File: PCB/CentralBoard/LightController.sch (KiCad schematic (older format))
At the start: 29 parts, among them P1 CONN_01X03, P2 CONN_01X10, P3 CONN_01X03, P4 CONN_01X10, P5 CONN_01X03, SW1 SW_DIP_x06, U1 LM317_3PinPackage, U2 NCP551, U3 PCA9685

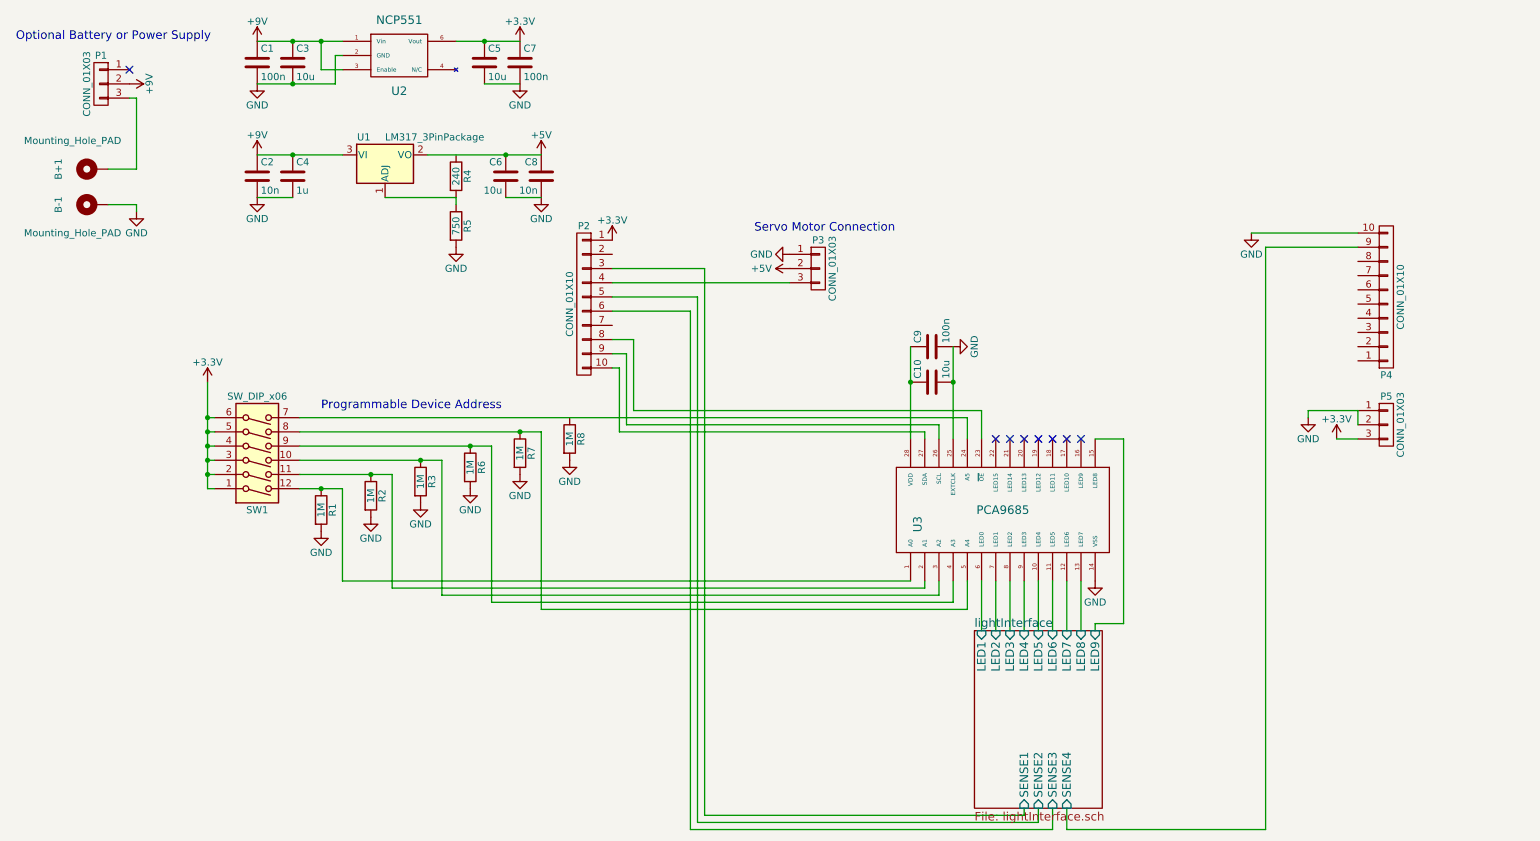
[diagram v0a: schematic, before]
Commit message: Created project specific footprint library. Placed all components. Started traces.
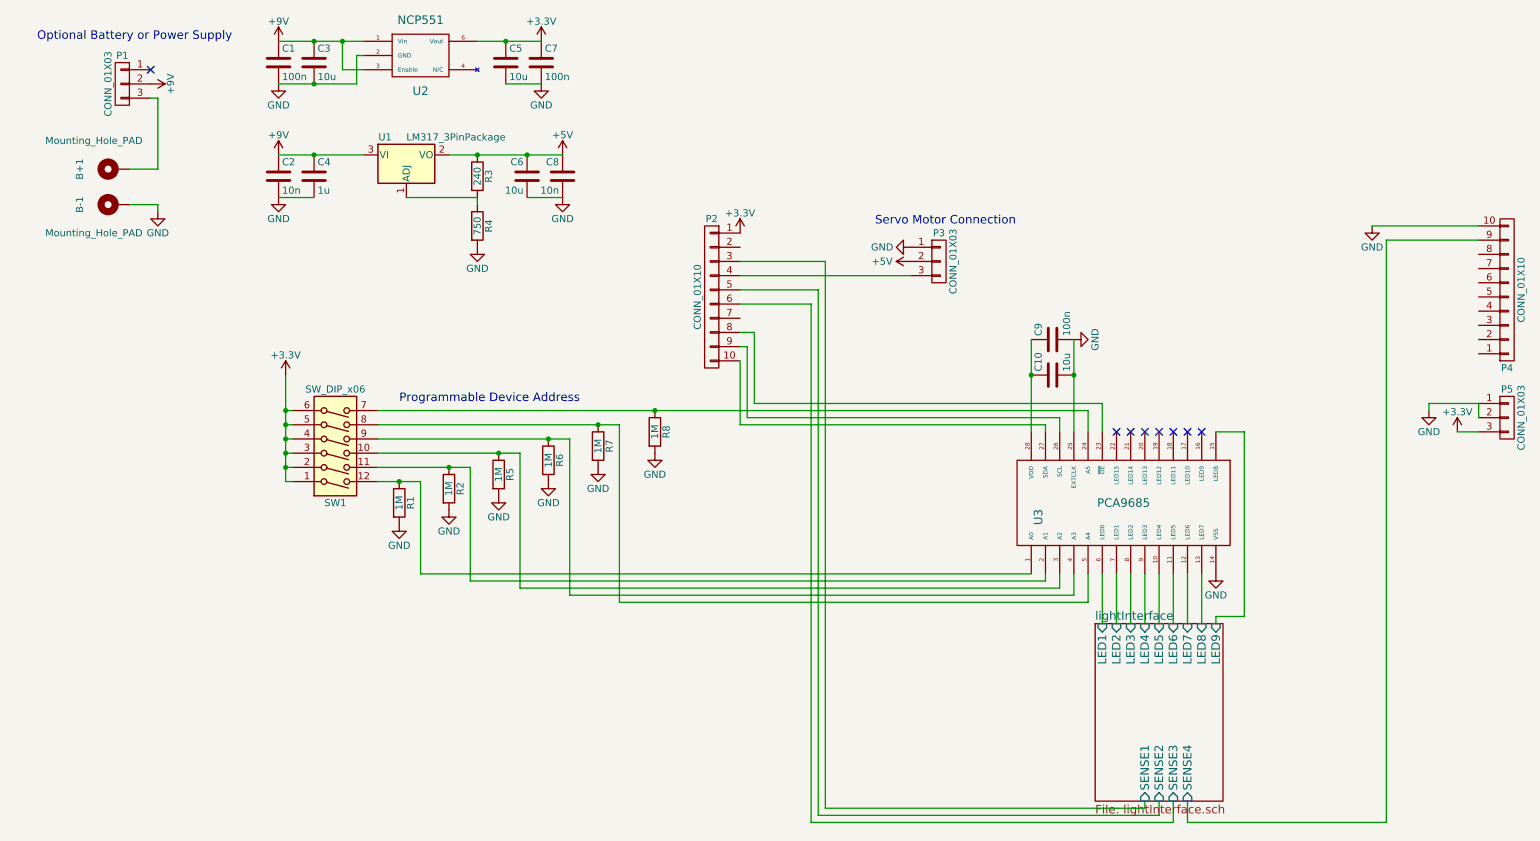
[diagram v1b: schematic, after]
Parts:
- C1, C10, C2, C3, C4, C5, C6, C7, C8, C9: footprint Capacitors_SMD:C_0805 -> Capacitors_SMD:C_0603
- R1, R2, R6, R7, R8: footprint Resistors_SMD:R_0805 -> Resistors_SMD:R_0603
- R3: renamed from R4; footprint Resistors_SMD:R_0805 -> Resistors_SMD:R_0603
- R4: renamed from R5; footprint Resistors_SMD:R_0805 -> Resistors_SMD:R_0603
- R5: renamed from R3; footprint Resistors_SMD:R_0805 -> Resistors_SMD:R_0603
- SW1: footprint MyLib:DIP_SW_219-6LPST -> CentralBoardFootprints:DIP_SW_219-6LPST
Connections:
- net +5V: now also R3.1
- net at SW1.7, U3.24 (A5): now also R8.1
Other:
- moved on the sheet: B+1, B-1, C1, C10, C2, C3, C4, C5, C6, C7, C8, C9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
